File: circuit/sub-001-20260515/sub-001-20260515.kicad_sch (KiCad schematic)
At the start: 7 parts

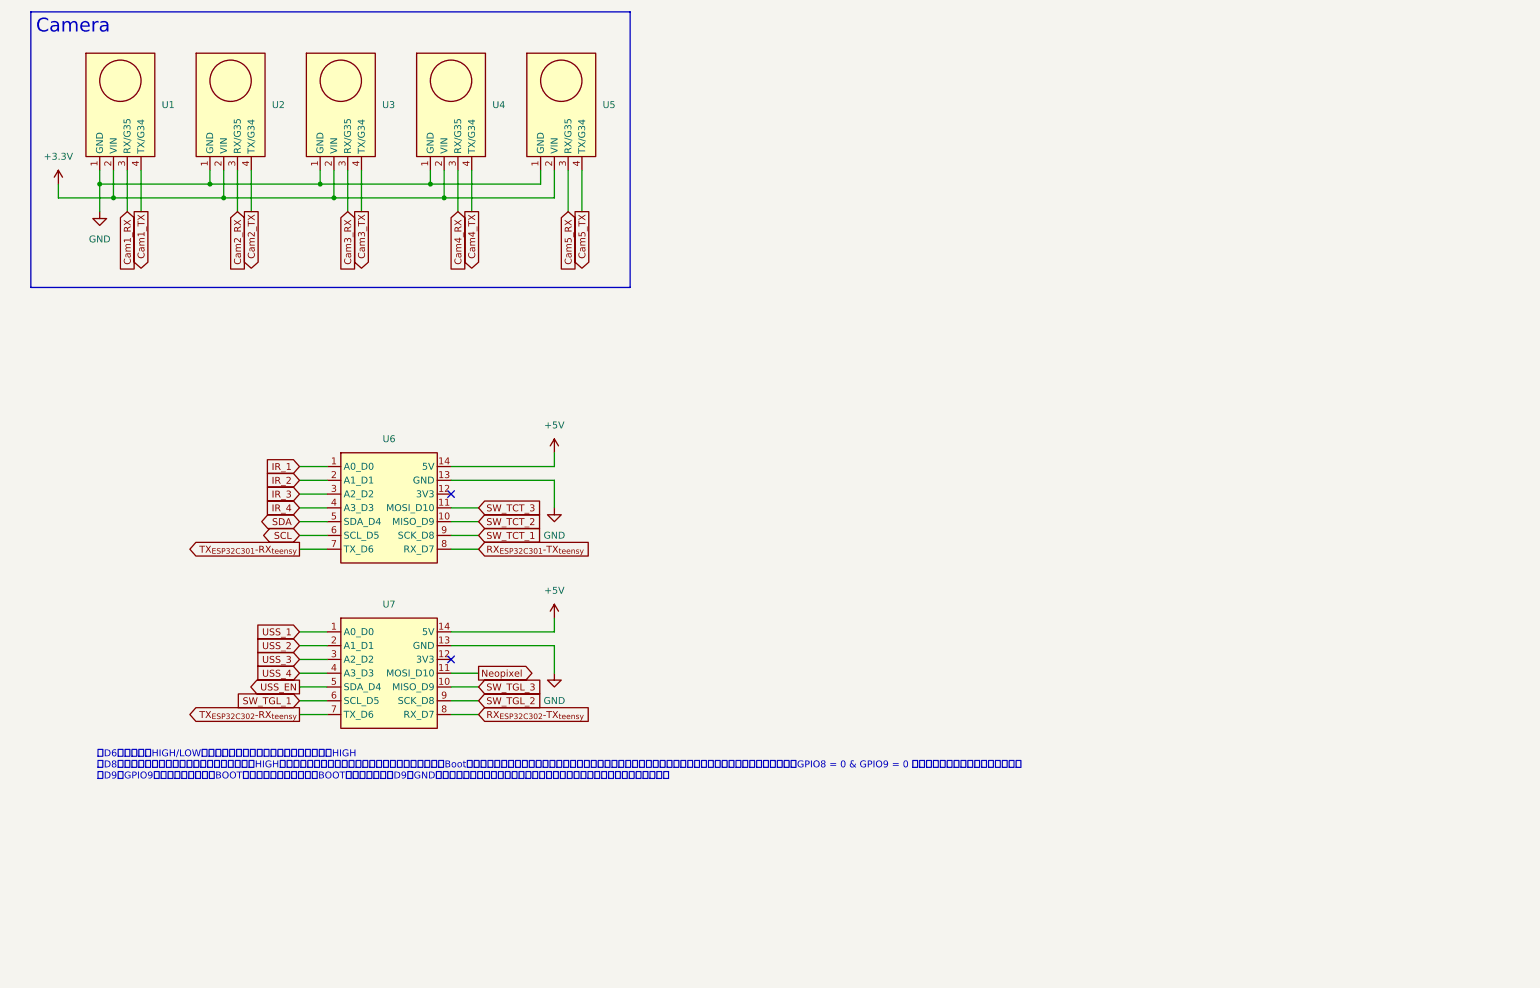
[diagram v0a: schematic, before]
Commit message: Update サブ基板完成した
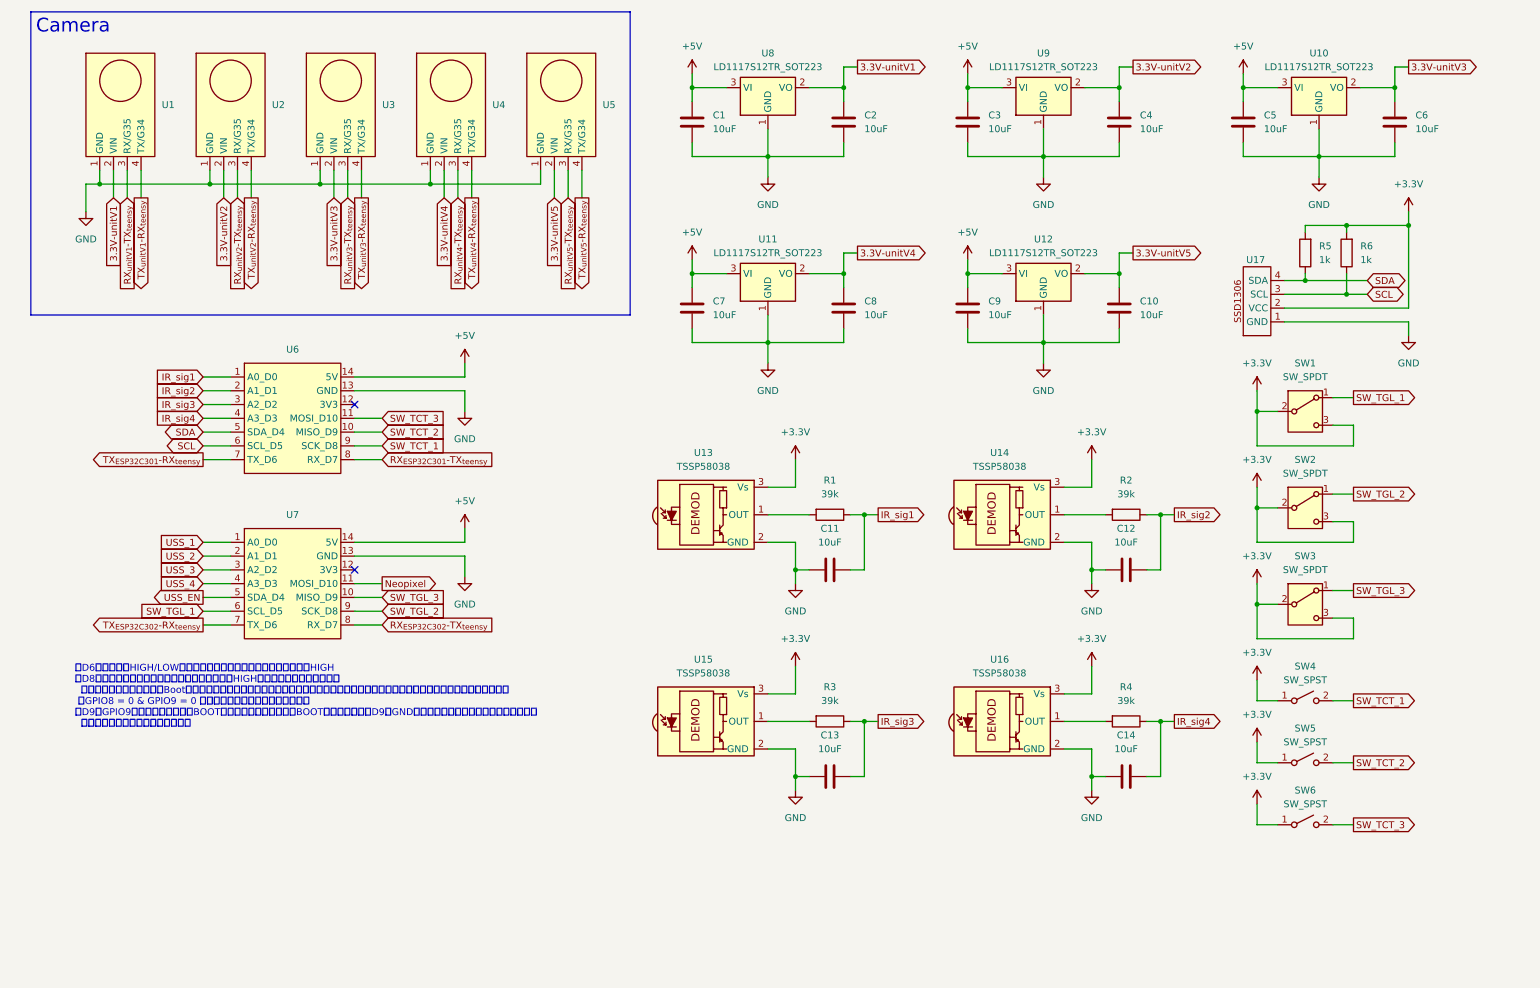
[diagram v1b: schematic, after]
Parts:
- added C1, C10, C11, C12, C13, C14, C2, C3, C4, C5, C6, C7, C8, C9: 10uF, symbol Device:C
- added R1, R2, R3, R4: 39k, symbol Device:R
- added R5, R6: 1k, symbol Device:R
- added SW1, SW2, SW3: SW_SPDT, symbol Switch:SW_SPDT
- added SW4, SW5, SW6: SW_SPST, symbol Switch:SW_SPST
- added U10, U11, U12, U8, U9: LD1117S12TR_SOT223, Package_TO_SOT_SMD:SOT-223-3_TabPin2, symbol Regulator_Linear:LD1117S12TR_SOT223
- added U13, U14, U15, U16: TSSP58038, OptoDevice:Vishay_MINICAST-3Pin, symbol Sensor_Proximity:TSSP58038
- added U17: (no value), symbol @Thrive_symbol_sub:SSD1306
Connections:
- net +3.3V: now also R5.2, R6.2, SW1.2 (B), SW1.3 (C), SW2.2 (B), SW2.3 (C), SW3.2 (B), SW3.3 (C), SW4.1 (A), SW5.1 (A), SW6.1 (A), U13.3 (Vs), U14.3 (Vs), U15.3 (Vs), U16.3 (Vs), U17.2 (VCC); no longer U1.2 (VIN), U2.2 (VIN), U3.2 (VIN), U4.2 (VIN), U5.2 (VIN)
- net +5V: now also C1.1, C3.1, C5.1, C7.1, C9.1, U10.3 (VI), U11.3 (VI), U12.3 (VI), U8.3 (VI), U9.3 (VI)
- net GND: now also C1.2, C10.2, C11.1, C12.1, C13.1, C14.1, C2.2, C3.2, C4.2, C5.2, C6.2, C7.2, C8.2, C9.2, U10.1 (GND), U11.1 (GND), U12.1 (GND), U13.2 (GND), U14.2 (GND), U15.2 (GND), U16.2 (GND), U17.1 (GND), U8.1 (GND), U9.1 (GND)
- net SCL: now also R6.1, U17.3 (SCL)
- net SDA: now also R5.1, U17.4 (SDA)
- net SW_TCT_1: now also SW4.2 (B)
- net SW_TCT_2: now also SW5.2 (B)
- net SW_TCT_3: now also SW6.2 (B)
- net SW_TGL_1: now also SW1.1 (A)
- net SW_TGL_2: now also SW2.1 (A)
- net SW_TGL_3: now also SW3.1 (A)
- net Cam1_RX renamed RX_{unitV1}-TX_{teensy}
- net Cam1_TX renamed TX_{unitV1}-RX_{teensy}
- net Cam2_RX renamed RX_{unitV2}-TX_{teensy}
- net Cam2_TX renamed TX_{unitV2}-RX_{teensy}
- net Cam3_RX renamed RX_{unitV3}-TX_{teensy}
- net Cam3_TX renamed TX_{unitV3}-RX_{teensy}
- net Cam4_RX renamed RX_{unitV4}-TX_{teensy}
- net Cam4_TX renamed TX_{unitV4}-RX_{teensy}
- net Cam5_RX renamed RX_{unitV5}-TX_{teensy}
- net Cam5_TX renamed TX_{unitV5}-RX_{teensy}
- net IR_1 renamed IR_sig1
- net IR_sig1: now also C11.2, R1.1
- net IR_2 renamed IR_sig2
- net IR_sig2: now also C12.2, R2.1
- net IR_3 renamed IR_sig3
- net IR_sig3: now also C13.2, R3.1
- net IR_4 renamed IR_sig4
- net IR_sig4: now also C14.2, R4.1
- new net: R2.2, U14.1 (OUT)
- new net: R4.2, U16.1 (OUT)
- new net: R1.2, U13.1 (OUT)
- new net: R3.2, U15.1 (OUT)
- new net 3.3V-unitV1: C2.1, U1.2 (VIN), U8.2 (VO)
- new net 3.3V-unitV2: C4.1, U2.2 (VIN), U9.2 (VO)
- new net 3.3V-unitV3: C6.1, U10.2 (VO), U3.2 (VIN)
- new net 3.3V-unitV4: C8.1, U11.2 (VO), U4.2 (VIN)
- new net 3.3V-unitV5: C10.1, U12.2 (VO), U5.2 (VIN)
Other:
- note added: "・D6は起動時にHIGH/LOWしてしまい、通信していない待機時は常にHIGH ・D8はプログラムの書き込みモードにした際に、HIGHになっている必要がある。 書き込みモードへの移行（Bootボタンを押しながらリセットする）を行う場合は、プルアップ抵抗をつけておくのがベターだそうです。 （GPIO8 = 0 & GPIO9 = 0 になると予期せぬ動きをする模様） ・D9はGPIO9とプルアップ抵抗、BOOTボタンに繋がっており、BOOTボタンを押すとD9がGNDに接続してしまうため、用途は限定的。 スイッチ入力に使うのがおすすめ。"
- note removed: "・D6は起動時にHIGH/LOWしてしまい、通信していない待機時は常にHIGH ・D8はプログラムの書き込みモードにした際に、HIGHになっている必要がある。書き込みモードへの移行（Bootボタンを押しながらリセットする）を行う場合は、プルアップ抵抗をつけておくのがベターだそうです。（GPIO8 = 0 & GPIO9 = 0 になると予期せぬ動きをする模様） ・D9はGPIO9とプルアップ抵抗、BOOTボタンに繋がっており、BOOTボタンを押すとD9がGNDに接続してしまうため、用途は限定的。スイッチ入力に使うのがおすすめ。"
- moved on the sheet: U6, U7

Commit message: Update サブ基板寺田DR後
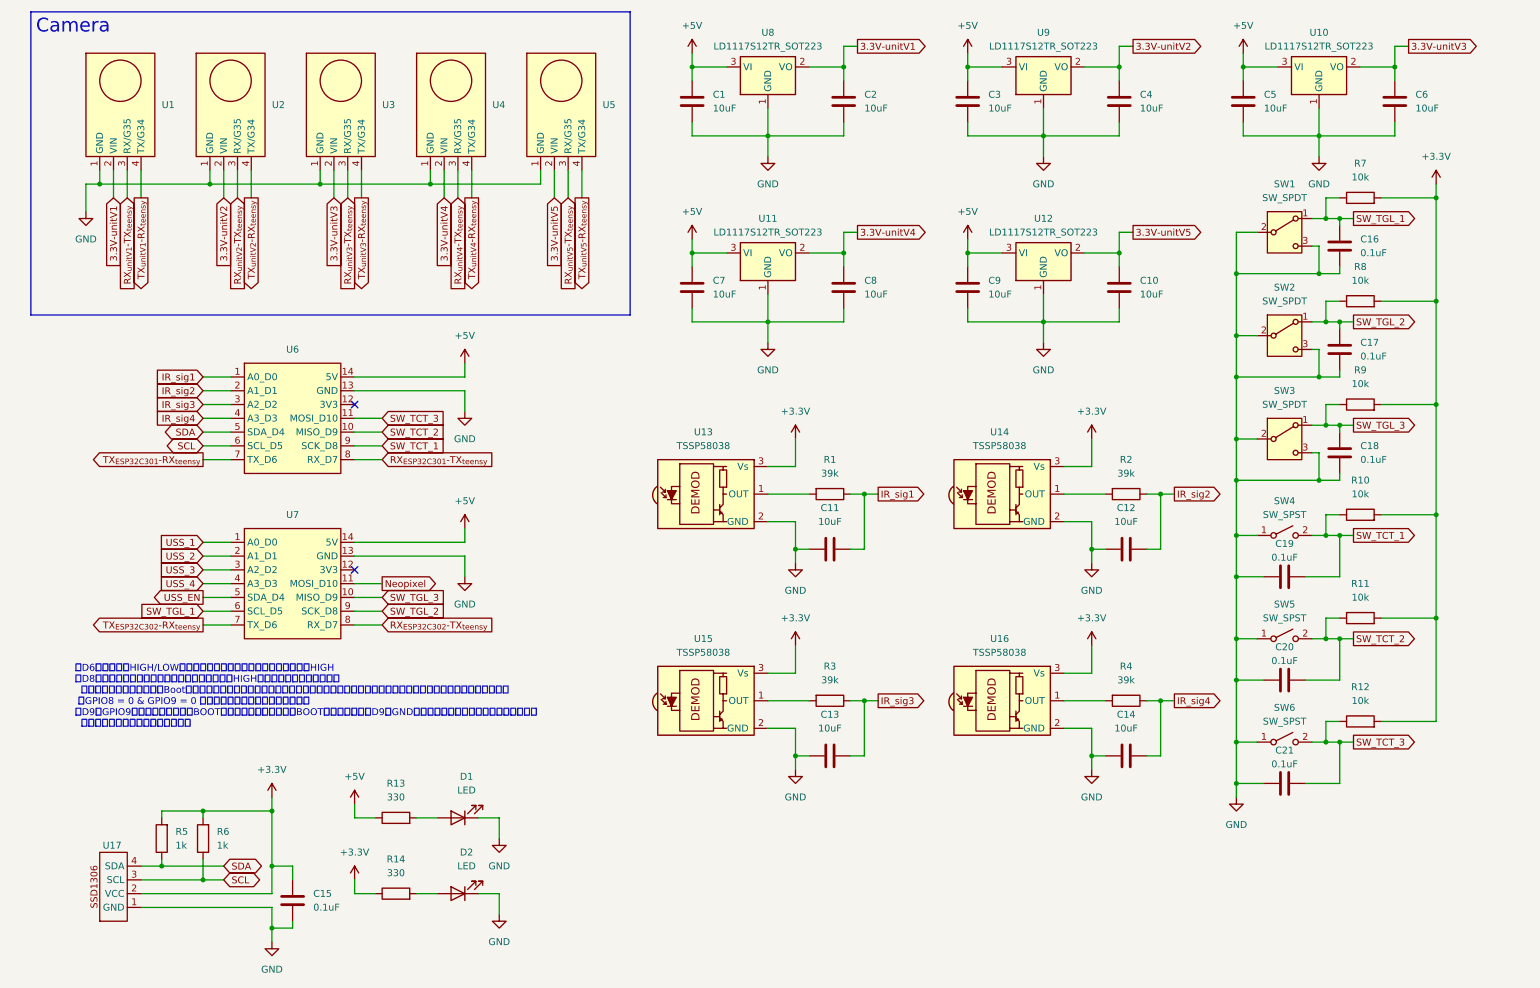
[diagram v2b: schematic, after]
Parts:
- added C15, C16, C17, C18, C19, C20, C21: 0.1uF, symbol Device:C
- added D1, D2: LED, symbol Device:LED
- added R10, R11, R12, R7, R8, R9: 10k, symbol Device:R
- added R13, R14: 330, symbol Device:R
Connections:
- net +3.3V: now also C15.1, R10.2, R11.2, R12.2, R14.1, R7.2, R8.2, R9.2; no longer SW1.2 (B), SW1.3 (C), SW2.2 (B), SW2.3 (C), SW3.2 (B), SW3.3 (C), SW4.1 (A), SW5.1 (A), SW6.1 (A)
- net +5V: now also R13.1
- net GND: now also SW1.2 (B), SW1.3 (C), SW2.2 (B), SW2.3 (C), SW3.2 (B), SW3.3 (C), SW4.1 (A), SW5.1 (A), SW6.1 (A), C15.2, C16.2, C17.2, C18.2, C19.2, C20.2, C21.2, D1.1 (K), D2.1 (K)
- net SW_TCT_1: now also C19.1, R10.1
- net SW_TCT_2: now also C20.1, R11.1
- net SW_TCT_3: now also C21.1, R12.1
- net SW_TGL_1: now also C16.1, R7.1
- net SW_TGL_2: now also C17.1, R8.1
- net SW_TGL_3: now also C18.1, R9.1
- new net: D2.2 (A), R14.2
- new net: D1.2 (A), R13.2
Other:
- moved on the sheet: C1, C10, C11, C12, C13, C14, C2, C3, C4, C5, C6, C7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
